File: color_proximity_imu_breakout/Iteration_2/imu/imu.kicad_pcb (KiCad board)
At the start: 2 copper layers, 13 x 20 mm, 15 parts, among them J1 Conn_01x10, J2 Conn_01x10, U6 ICM-20602

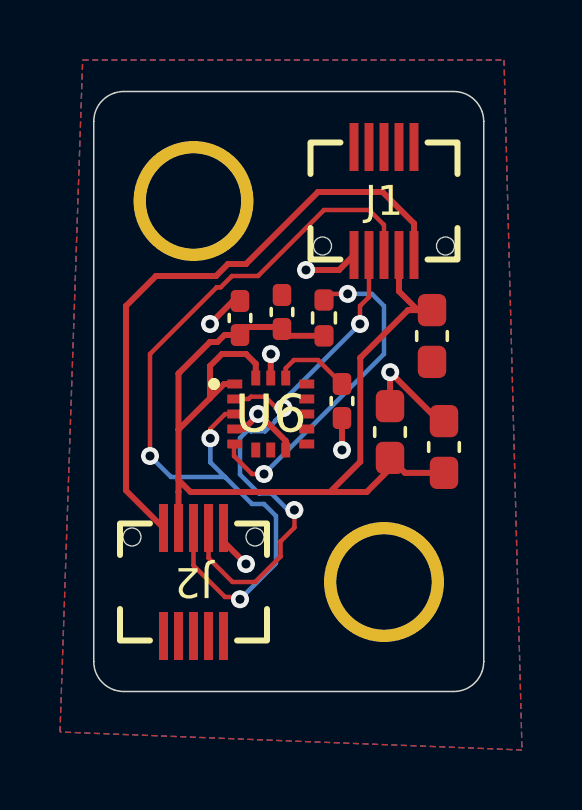
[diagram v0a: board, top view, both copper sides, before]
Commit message: updated production files
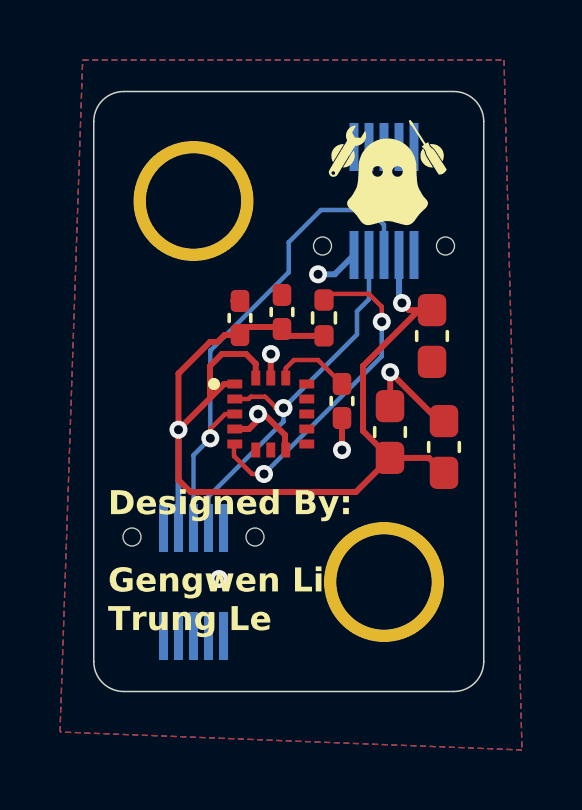
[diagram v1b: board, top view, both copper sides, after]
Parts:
- removed the G*** at (146.6, 136.8)
- removed the G*** at (144.2, 142.2)
- G***: moved to F.Cu
- J1, J2: moved to B.Cu
- moved G*** 12.9 mm to (148.9, 127.4), turned to 0 degrees
- turned C1 to -90 degrees
- turned C2 to 90 degrees
- turned J1 to 180 degrees
- turned J2 to 0 degrees
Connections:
- C1 pad 1: GND -> +3.3V
- C1 pad 2: +3.3V -> GND
- C2 pad 1: GND -> +3.3V
- C2 pad 2: +3.3V -> GND
- J1 pad 10: +5V -> GND
- J1 pad 6: GND -> unconnected-(J1-Pin_6-Pad6)
- J1 pad 7: /scl -> +3.3V
- J1 pad 9: +3.3V -> /scl
- J2 pad 10: +5V -> GND
- J2 pad 6: GND -> unconnected-(J2-Pin_6-Pad6)
- J2 pad 7: /scl -> +3.3V
- J2 pad 9: +3.3V -> /scl
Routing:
- net +5V: track 20.6 -> 0.00 mm
- net /sda: track 28.8 -> 17.0 mm, vias 3 -> 1
- net /scl: track 19.5 -> 13.2 mm, vias 3 -> 1
- net GND: track 13.1 -> 10.00 mm, vias 7 -> 6
- net +3.3V: track 36.7 -> 37.2 mm, vias 0 -> 2
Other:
- board text added: "Designed By: Gengwen Li Trung Le"
- board text removed: "Designed By Gengwen Li Trung Le"
